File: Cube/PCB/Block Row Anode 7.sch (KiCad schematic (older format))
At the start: 10 parts

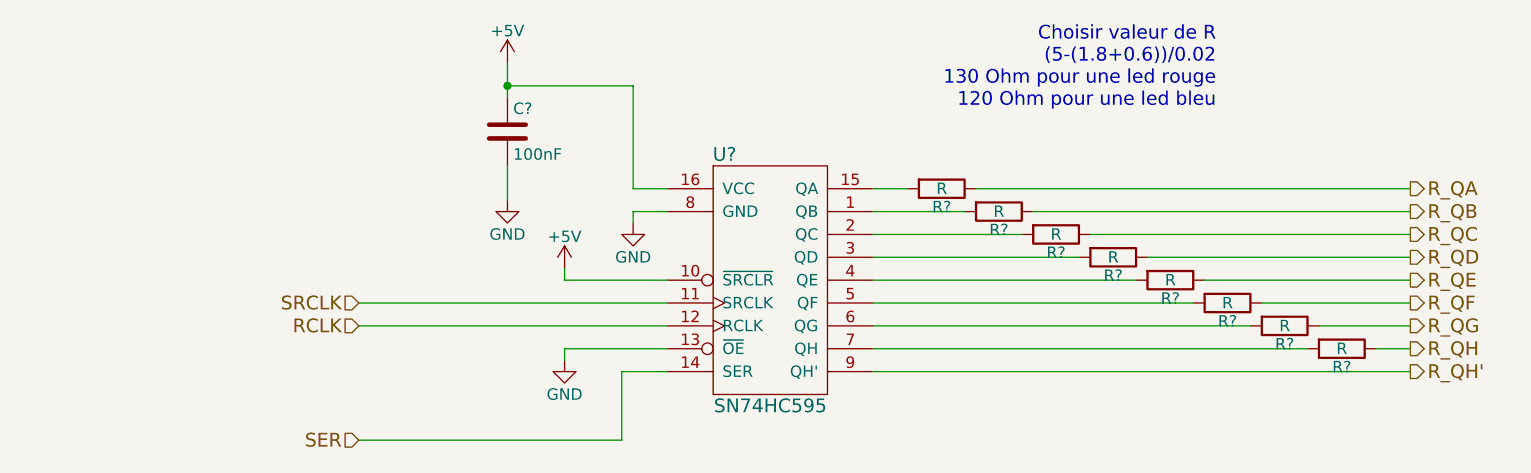
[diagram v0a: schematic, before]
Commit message: Update
Update
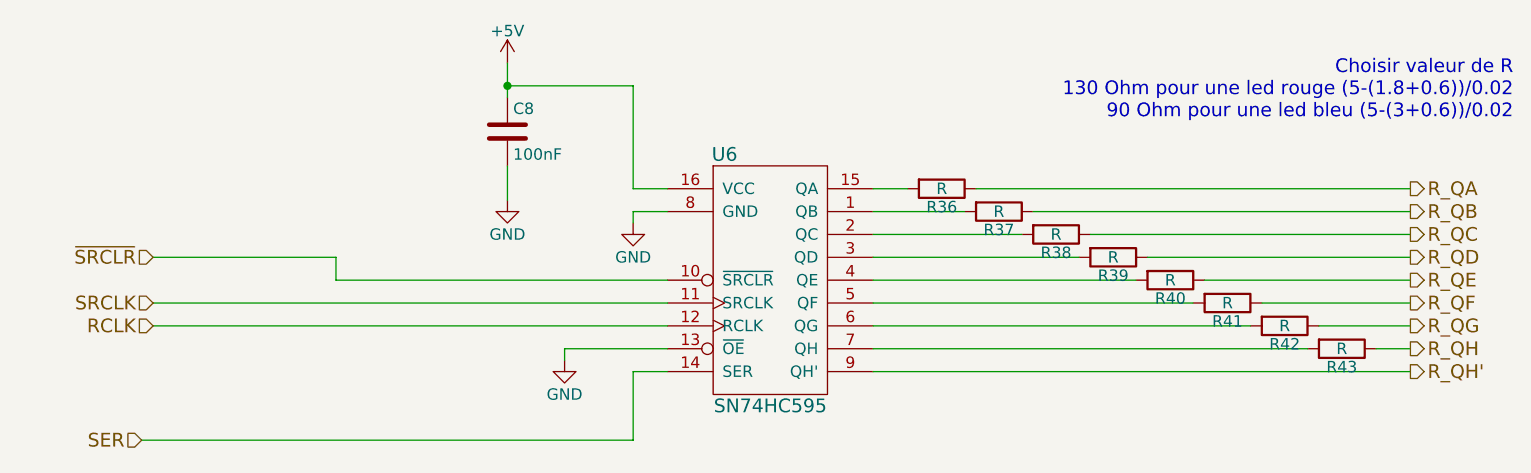
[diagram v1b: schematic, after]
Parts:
- removed C?: 100nF, symbol C
- removed R? (x8): R, symbol R
- removed U?: SN74HC595, symbol SN74HC595
- added C8: 100nF, symbol C
- added R36, R37, R38, R39, R40, R41, R42, R43: R, symbol R
- added U6: SN74HC595, symbol SN74HC595
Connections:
- net +5V: now also C8.1, U6.16 (VCC)
- net GND: now also C8.2, U6.13 (~OE), U6.8 (GND)
- net RCLK: now also U6.12 (RCLK)
- net R_QA: now also R36.1
- net R_QB: now also R37.1
- net R_QC: now also R38.1
- net R_QD: now also R39.1
- net R_QE: now also R40.1
- net R_QF: now also R41.1
- net R_QG: now also R42.1
- net R_QH: now also R43.1
- net R_QH': now also U6.9 (QH')
- net SER: now also U6.14 (SER)
- net SRCLK: now also U6.11 (SRCLK)
- new net: R37.2, U6.1 (QB)
- new net: R36.2, U6.15 (QA)
- new net: R38.2, U6.2 (QC)
- new net: R39.2, U6.3 (QD)
- new net: R40.2, U6.4 (QE)
- new net: R41.2, U6.5 (QF)
- new net: R42.2, U6.6 (QG)
- new net: R43.2, U6.7 (QH)
- new net ~SRCLR: U6.10 (~SRCLR)
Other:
- note added: "Choisir valeur de R\n130 Ohm pour une led rouge (5-(1.8+0.6))/0.02\n90 Ohm pour une led bleu (5-(3+0.6))/0.02"
- note removed: "Choisir valeur de R\n(5-(1.8+0.6))/0.02\n130 Ohm pour une led rouge\n120 Ohm pour une led bleu"
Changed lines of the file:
@@
 LIBS:valves
 LIBS:alex-library
+LIBS:Cube-8x8x8-512_LEDS-cache
 EELAYER 25 0
 EELAYER END
 $Descr A4 11693 8268
 encoding utf-8
-Sheet 5 5
+Sheet 8 12
 Title ""
 Date ""
@@
 $EndDescr
 $Comp
-L SN74HC595 U?
-U 1 1 5B2235DE
+L SN74HC595 U6
+U 1 1 5B236688
 P 4900 3650
-AR Path="/5B22355E/5B2235D3/5B2235DE" Ref="U?"  Part="1"
-AR Path="/5B22355E/5B22654D/5B2235DE" Ref="U?"  Part="1"
-F 0 "U?" H 4700 4200 60  0000 C CNN
+F 0 "U6" H 4700 4200 60  0000 C CNN
 F 1 "SN74HC595" H 4900 3100 60  0000 C CNN
 F 2 "" H 5250 3550 60  0001 C CNN
@@
 $EndComp
 $Comp
-L C C?
-U 1 1 5B223645
+L C C8
+U 1 1 5B236689
 P 3750 3000
-AR Path="/5B22355E/5B2235D3/5B223645" Ref="C?"  Part="1"
-AR Path="/5B22355E/5B22654D/5B223645" Ref="C?"  Part="1"
-F 0 "C?" H 3775 3100 50  0000 L CNN
+F 0 "C8" H 3775 3100 50  0000 L CNN
 F 1 "100nF" H 3775 2900 50  0000 L CNN
 F 2 "" H 3788 2850 50  0001 C CNN
@@
 $EndComp
 $Comp
-L +5V #PWR?
-U 1 1 5B223671
+L +5V #PWR30
+U 1 1 5B23668A
 P 3750 2700
-AR Path="/5B22355E/5B2235D3/5B223671" Ref="#PWR?"  Part="1"
-AR Path="/5B22355E/5B22654D/5B223671" Ref="#PWR?"  Part="1"
-F 0 "#PWR?" H 3750 2550 50  0001 C CNN
+F 0 "#PWR30" H 3750 2550 50  0001 C CNN
 F 1 "+5V" H 3750 2840 50  0000 C CNN
 F 2 "" H 3750 2700 50  0001 C CNN
@@
 $EndComp
 $Comp
-L GND #PWR?
-U 1 1 5B223689
+L GND #PWR31
+U 1 1 5B23668B
 P 3750 3300
-AR Path="/5B22355E/5B2235D3/5B223689" Ref="#PWR?"  Part="1"
-AR Path="/5B22355E/5B22654D/5B223689" Ref="#PWR?"  Part="1"
-F 0 "#PWR?" H 3750 3050 50  0001 C CNN
+F 0 "#PWR31" H 3750 3050 50  0001 C CNN
 F 1 "GND" H 3750 3150 50  0000 C CNN
 F 2 "" H 3750 3300 50  0001 C CNN
@@
 $EndComp
 $Comp
-L GND #PWR?
-U 1 1 5B2236C5
+L GND #PWR33
+U 1 1 5B23668C
 P 4300 3400
-AR Path="/5B22355E/5B2235D3/5B2236C5" Ref="#PWR?"  Part="1"
-AR Path="/5B22355E/5B22654D/5B2236C5" Ref="#PWR?"  Part="1"
-F 0 "#PWR?" H 4300 3150 50  0001 C CNN
+F 0 "#PWR33" H 4300 3150 50  0001 C CNN
 F 1 "GND" H 4300 3250 50  0000 C CNN
 F 2 "" H 4300 3400 50  0001 C CNN
@@
 $EndComp
 $Comp
-L +5V #PWR?
-U 1 1 5B223752
-P 4000 3600
-F 0 "#PWR?" H 4000 3450 50  0001 C CNN
-F 1 "+5V" H 4000 3740 50  0000 C CNN
-F 2 "" H 4000 3600 50  0001 C CNN
-F 3 "" H 4000 3600 50  0001 C CNN
-	1    4000 3600
-	1    0    0    -1
-$EndComp
-$Comp
-L GND #PWR?
-U 1 1 5B2237AC
+L GND #PWR32
+U 1 1 5B23668D
 P 4000 4000
-F 0 "#PWR?" H 4000 3750 50  0001 C CNN
+F 0 "#PWR32" H 4000 3750 50  0001 C CNN
 F 1 "GND" H 4000 3850 50  0000 C CNN
 F 2 "" H 4000 4000 50  0001 C CNN
@@
 	1    0    0    -1
 $EndComp
-Text HLabel 3100 3750 0    60   Input ~ 0
+Text HLabel 2200 3750 0    60   Input ~ 0
 SRCLK
-Text HLabel 3100 3850 0    60   Input ~ 0
+Text HLabel 2200 3850 0    60   Input ~ 0
 RCLK
-Text HLabel 3100 4350 0    60   Input ~ 0
+Text HLabel 2150 4350 0    60   Input ~ 0
 SER
 Text HLabel 7700 3250 2    60   Output ~ 0
@@
 R_QH'
 $Comp
-L R R?
-U 1 1 5B2238E0
+L R R36
+U 1 1 5B23668E
 P 5650 3250
-AR Path="/5B22355E/5B2235D3/5B2238E0" Ref="R?"  Part="1"
-AR Path="/5B22355E/5B22654D/5B2238E0" Ref="R?"  Part="1"
-F 0 "R?" V 5730 3250 50  0000 C CNN
+F 0 "R36" V 5730 3250 50  0000 C CNN
 F 1 "R" V 5650 3250 50  0000 C CNN
 F 2 "" V 5580 3250 50  0001 C CNN
@@
 $EndComp
 $Comp
-L R R?
-U 1 1 5B223906
+L R R37
+U 1 1 5B23668F
 P 5900 3350
-AR Path="/5B22355E/5B2235D3/5B223906" Ref="R?"  Part="1"
-AR Path="/5B22355E/5B22654D/5B223906" Ref="R?"  Part="1"
-F 0 "R?" V 5980 3350 50  0000 C CNN
+F 0 "R37" V 5980 3350 50  0000 C CNN
 F 1 "R" V 5900 3350 50  0000 C CNN
 F 2 "" V 5830 3350 50  0001 C CNN
@@
 $EndComp
 $Comp
-L R R?
-U 1 1 5B223932
+L R R38
+U 1 1 5B236690
 P 6150 3450
-AR Path="/5B22355E/5B2235D3/5B223932" Ref="R?"  Part="1"
-AR Path="/5B22355E/5B22654D/5B223932" Ref="R?"  Part="1"
-F 0 "R?" V 6230 3450 50  0000 C CNN
+F 0 "R38" V 6230 3450 50  0000 C CNN
 F 1 "R" V 6150 3450 50  0000 C CNN
 F 2 "" V 6080 3450 50  0001 C CNN
@@
 $EndComp
 $Comp
-L R R?
-U 1 1 5B2239C6
+L R R39
+U 1 1 5B236691
 P 6400 3550
-AR Path="/5B22355E/5B2235D3/5B2239C6" Ref="R?"  Part="1"
-AR Path="/5B22355E/5B22654D/5B2239C6" Ref="R?"  Part="1"
-F 0 "R?" V 6480 3550 50  0000 C CNN
+F 0 "R39" V 6480 3550 50  0000 C CNN
 F 1 "R" V 6400 3550 50  0000 C CNN
 F 2 "" V 6330 3550 50  0001 C CNN
@@
 $EndComp
 $Comp
-L R R?
-U 1 1 5B2239FA
+L R R40
+U 1 1 5B236692
 P 6650 3650
-AR Path="/5B22355E/5B2235D3/5B2239FA" Ref="R?"  Part="1"
-AR Path="/5B22355E/5B22654D/5B2239FA" Ref="R?"  Part="1"
-F 0 "R?" V 6730 3650 50  0000 C CNN
+F 0 "R40" V 6730 3650 50  0000 C CNN
 F 1 "R" V 6650 3650 50  0000 C CNN
 F 2 "" V 6580 3650 50  0001 C CNN
@@
 $EndComp
 $Comp
-L R R?
-U 1 1 5B223A31
+L R R41
+U 1 1 5B236693
 P 6900 3750
-AR Path="/5B22355E/5B2235D3/5B223A31" Ref="R?"  Part="1"
-AR Path="/5B22355E/5B22654D/5B223A31" Ref="R?"  Part="1"
-F 0 "R?" V 6980 3750 50  0000 C CNN
+F 0 "R41" V 6980 3750 50  0000 C CNN
 F 1 "R" V 6900 3750 50  0000 C CNN
 F 2 "" V 6830 3750 50  0001 C CNN
@@
 $EndComp
 $Comp
-L R R?
-U 1 1 5B223B39
+L R R42
+U 1 1 5B236694
 P 7150 3850
-AR Path="/5B22355E/5B2235D3/5B223B39" Ref="R?"  Part="1"
-AR Path="/5B22355E/5B22654D/5B223B39" Ref="R?"  Part="1"
-F 0 "R?" V 7230 3850 50  0000 C CNN
+F 0 "R42" V 7230 3850 50  0000 C CNN
 F 1 "R" V 7150 3850 50  0000 C CNN
 F 2 "" V 7080 3850 50  0001 C CNN
@@
 Connection ~ 3750 2800
 Wire Wire Line
-	4000 3600 4000 3650
-Wire Wire Line
-	4000 3650 4450 3650
-Wire Wire Line
 	4450 3950 4000 3950
 Wire Wire Line
@@
 	5350 3850 7000 3850
 $Comp
-L R R?
-U 1 1 5B2240C8
+L R R43
+U 1 1 5B236695
 P 7400 3950
-F 0 "R?" V 7480 3950 50  0000 C CNN
+F 0 "R43" V 7480 3950 50  0000 C CNN
 F 1 "R" V 7400 3950 50  0000 C CNN
 F 2 "" V 7330 3950 50  0001 C CNN
@@
 Wire Wire Line
 	7550 3950 7700 3950
-Wire Wire Line
-	3100 3750 4450 3750
-Wire Wire Line
-	3100 3850 4450 3850
-Wire Wire Line
-	4450 4050 4250 4050
-Wire Wire Line
-	4250 4050 4250 4350
-Wire Wire Line
-	4250 4350 3100 4350
-Text Notes 6850 2900 2    60   ~ 0
-Choisir valeur de R\n(5-(1.8+0.6))/0.02\n130 Ohm pour une led rouge\n120 Ohm pour une led bleu
+Text Notes 8150 2950 2    60   ~ 0
+Choisir valeur de R\n130 Ohm pour une led rouge (5-(1.8+0.6))/0.02\n90 Ohm pour une led bleu (5-(3+0.6))/0.02
+Wire Wire Line
+	2200 3750 4450 3750
+Wire Wire Line
+	2200 3850 4450 3850
+Wire Wire Line
+	2150 4350 4300 4350
+Wire Wire Line
+	4300 4350 4300 4050
+Wire Wire Line
+	4300 4050 4450 4050
+Text HLabel 2200 3550 0    60   Input ~ 0
+~SRCLR
+Wire Wire Line
+	2200 3550 3000 3550
+Wire Wire Line
+	3000 3550 3000 3650
+Wire Wire Line
+	3000 3650 4450 3650
 $EndSCHEMATC

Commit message: Update project
Remove a image corrupted -_-
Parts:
- C8: footprint (none) -> alex-library:C-P_5.08-L_7.5-H_6-P_2.5
- R36, R37, R38, R39, R40, R41, R42, R43: footprint (none) -> alex-library:R_Axial_Long6.3mm_Dia2.5mm_Pas15.24mm_Horizontal
- U6: footprint (none) -> alex-library:DIP-16_W7.62mm_LongPads
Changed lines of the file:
@@
 F 0 "U6" H 4700 4200 60  0000 C CNN
 F 1 "SN74HC595" H 4900 3100 60  0000 C CNN
-F 2 "" H 5250 3550 60  0001 C CNN
+F 2 "alex-library:DIP-16_W7.62mm_LongPads" H 5250 3550 60  0001 C CNN
 F 3 "" H 5250 3550 60  0001 C CNN
 	1    4900 3650
@@
 F 0 "C8" H 3775 3100 50  0000 L CNN
 F 1 "100nF" H 3775 2900 50  0000 L CNN
-F 2 "" H 3788 2850 50  0001 C CNN
+F 2 "alex-library:C-P_5.08-L_7.5-H_6-P_2.5" H 3788 2850 50  0001 C CNN
 F 3 "" H 3750 3000 50  0001 C CNN
 	1    3750 3000
@@
 $EndComp
 $Comp
-L +5V #PWR30
+L +5V #PWR038
 U 1 1 5B23668A
 P 3750 2700
-F 0 "#PWR30" H 3750 2550 50  0001 C CNN
+F 0 "#PWR038" H 3750 2550 50  0001 C CNN
 F 1 "+5V" H 3750 2840 50  0000 C CNN
 F 2 "" H 3750 2700 50  0001 C CNN
@@
 $EndComp
 $Comp
-L GND #PWR31
+L GND #PWR039
 U 1 1 5B23668B
 P 3750 3300
-F 0 "#PWR31" H 3750 3050 50  0001 C CNN
+F 0 "#PWR039" H 3750 3050 50  0001 C CNN
 F 1 "GND" H 3750 3150 50  0000 C CNN
 F 2 "" H 3750 3300 50  0001 C CNN
@@
 $EndComp
 $Comp
-L GND #PWR33
+L GND #PWR040
 U 1 1 5B23668C
 P 4300 3400
-F 0 "#PWR33" H 4300 3150 50  0001 C CNN
+F 0 "#PWR040" H 4300 3150 50  0001 C CNN
 F 1 "GND" H 4300 3250 50  0000 C CNN
 F 2 "" H 4300 3400 50  0001 C CNN
@@
 $EndComp
 $Comp
-L GND #PWR32
+L GND #PWR041
 U 1 1 5B23668D
 P 4000 4000
-F 0 "#PWR32" H 4000 3750 50  0001 C CNN
+F 0 "#PWR041" H 4000 3750 50  0001 C CNN
 F 1 "GND" H 4000 3850 50  0000 C CNN
 F 2 "" H 4000 4000 50  0001 C CNN
@@
 F 0 "R36" V 5730 3250 50  0000 C CNN
 F 1 "R" V 5650 3250 50  0000 C CNN
-F 2 "" V 5580 3250 50  0001 C CNN
+F 2 "alex-library:R_Axial_Long6.3mm_Dia2.5mm_Pas15.24mm_Horizontal" V 5580 3250 50  0001 C CNN
 F 3 "" H 5650 3250 50  0001 C CNN
 	1    5650 3250
@@
 F 0 "R37" V 5980 3350 50  0000 C CNN
 F 1 "R" V 5900 3350 50  0000 C CNN
-F 2 "" V 5830 3350 50  0001 C CNN
+F 2 "alex-library:R_Axial_Long6.3mm_Dia2.5mm_Pas15.24mm_Horizontal" V 5830 3350 50  0001 C CNN
 F 3 "" H 5900 3350 50  0001 C CNN
 	1    5900 3350
@@
 F 0 "R38" V 6230 3450 50  0000 C CNN
 F 1 "R" V 6150 3450 50  0000 C CNN
-F 2 "" V 6080 3450 50  0001 C CNN
+F 2 "alex-library:R_Axial_Long6.3mm_Dia2.5mm_Pas15.24mm_Horizontal" V 6080 3450 50  0001 C CNN
 F 3 "" H 6150 3450 50  0001 C CNN
 	1    6150 3450
@@
 F 0 "R39" V 6480 3550 50  0000 C CNN
 F 1 "R" V 6400 3550 50  0000 C CNN
-F 2 "" V 6330 3550 50  0001 C CNN
+F 2 "alex-library:R_Axial_Long6.3mm_Dia2.5mm_Pas15.24mm_Horizontal" V 6330 3550 50  0001 C CNN
 F 3 "" H 6400 3550 50  0001 C CNN
 	1    6400 3550
@@
 F 0 "R40" V 6730 3650 50  0000 C CNN
 F 1 "R" V 6650 3650 50  0000 C CNN
-F 2 "" V 6580 3650 50  0001 C CNN
+F 2 "alex-library:R_Axial_Long6.3mm_Dia2.5mm_Pas15.24mm_Horizontal" V 6580 3650 50  0001 C CNN
 F 3 "" H 6650 3650 50  0001 C CNN
 	1    6650 3650
@@
 F 0 "R41" V 6980 3750 50  0000 C CNN
 F 1 "R" V 6900 3750 50  0000 C CNN
-F 2 "" V 6830 3750 50  0001 C CNN
+F 2 "alex-library:R_Axial_Long6.3mm_Dia2.5mm_Pas15.24mm_Horizontal" V 6830 3750 50  0001 C CNN
 F 3 "" H 6900 3750 50  0001 C CNN
 	1    6900 3750
@@
 F 0 "R42" V 7230 3850 50  0000 C CNN
 F 1 "R" V 7150 3850 50  0000 C CNN
-F 2 "" V 7080 3850 50  0001 C CNN
+F 2 "alex-library:R_Axial_Long6.3mm_Dia2.5mm_Pas15.24mm_Horizontal" V 7080 3850 50  0001 C CNN
 F 3 "" H 7150 3850 50  0001 C CNN
 	1    7150 3850
@@
 F 0 "R43" V 7480 3950 50  0000 C CNN
 F 1 "R" V 7400 3950 50  0000 C CNN
-F 2 "" V 7330 3950 50  0001 C CNN
+F 2 "alex-library:R_Axial_Long6.3mm_Dia2.5mm_Pas15.24mm_Horizontal" V 7330 3950 50  0001 C CNN
 F 3 "" H 7400 3950 50  0001 C CNN
 	1    7400 3950
